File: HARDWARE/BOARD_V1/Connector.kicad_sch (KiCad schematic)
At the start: 40 parts, among them J1 SFW15R-2STE1LF, J2 USB_C_Receptacle_USB2.0_16P, J3 47309-2651, J4 Conn_ARM_SWD_TagConnect_TC203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, J5 687108183722, Q1 BSS84AKQBZ

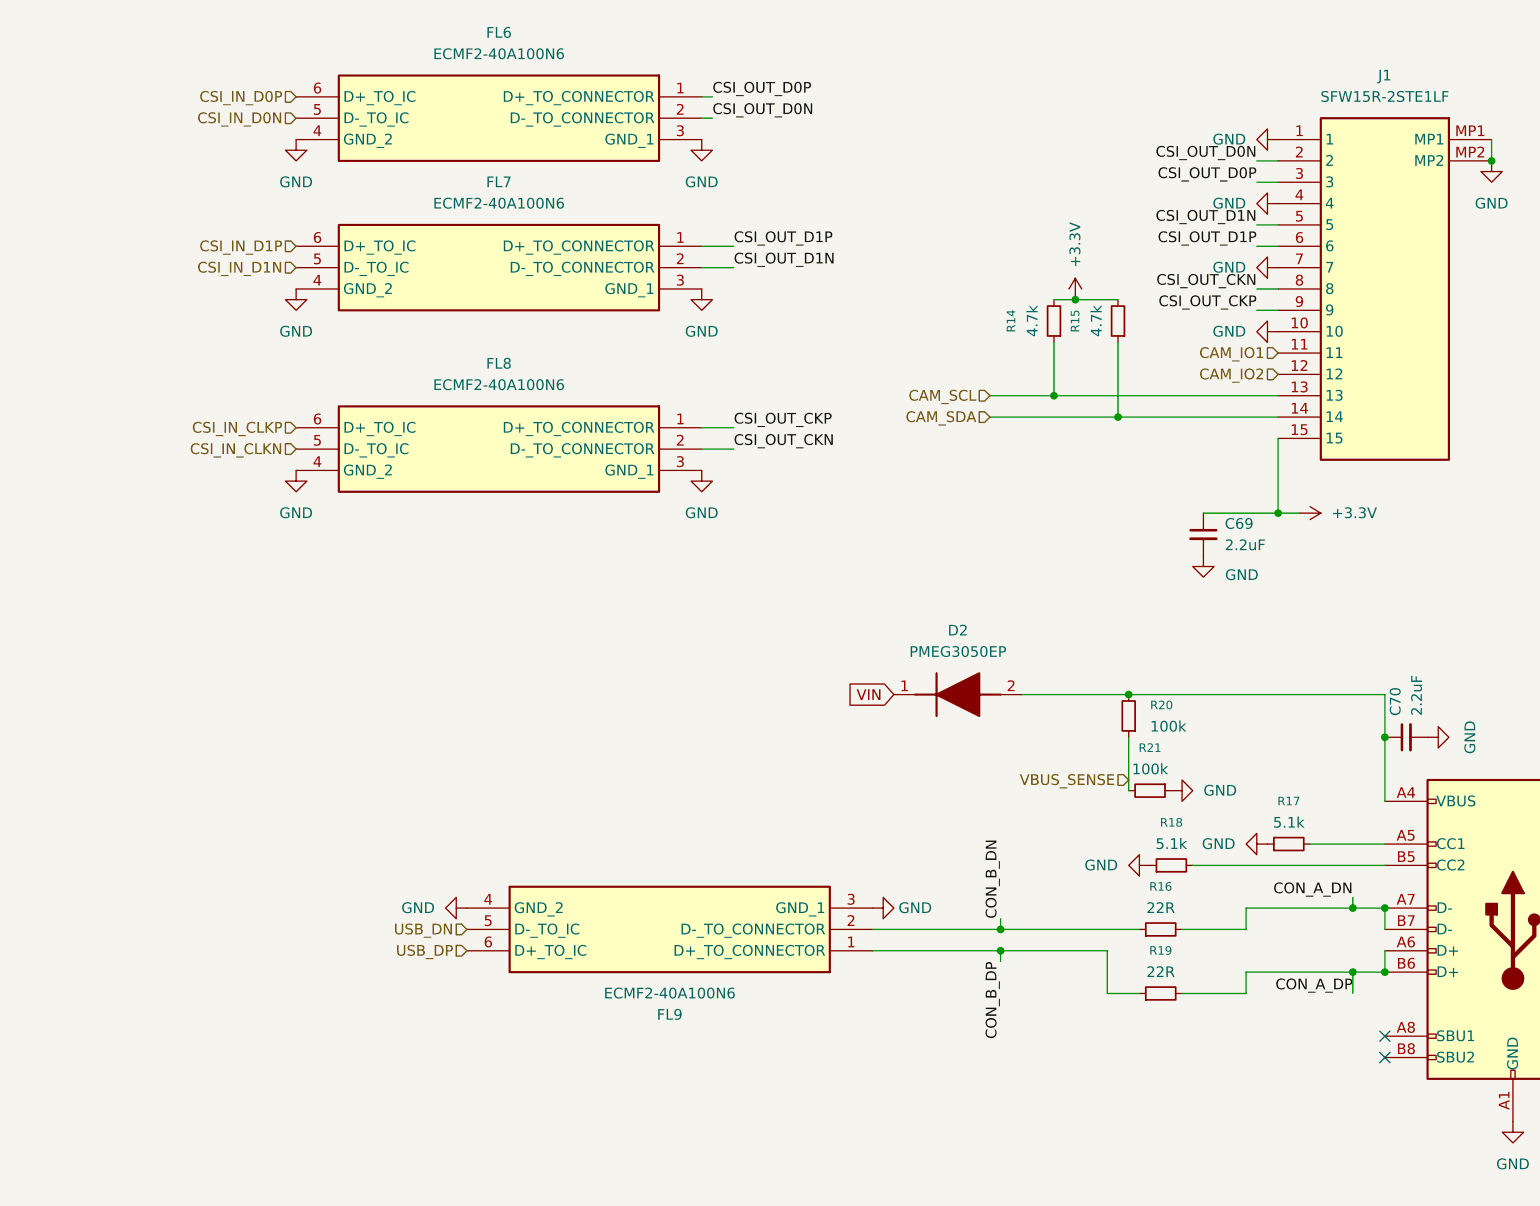
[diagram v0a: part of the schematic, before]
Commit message: up
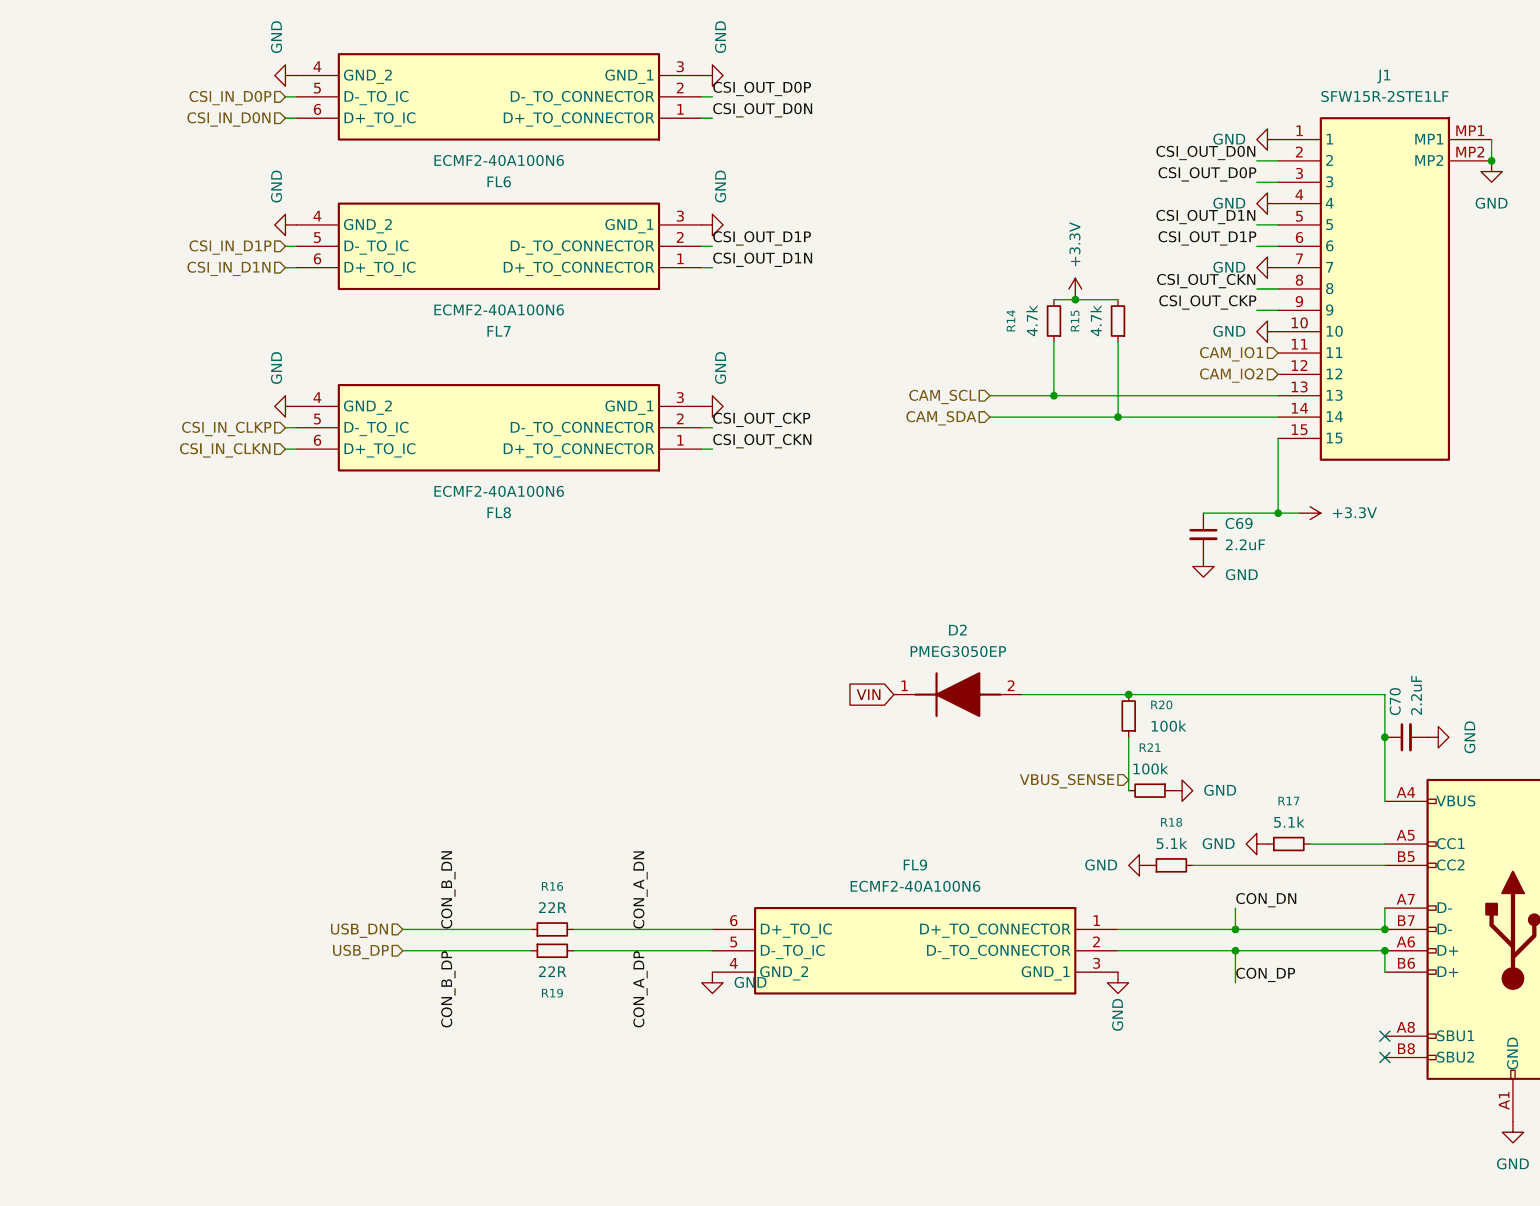
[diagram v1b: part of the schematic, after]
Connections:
- net CON_A_DN: now also FL9.6 (D+_TO_IC); no longer J2.A7 (D-), J2.B7 (D-)
- net CON_A_DP: now also FL9.5 (D-_TO_IC); no longer J2.A6 (D+), J2.B6 (D+)
- net CSI_IN_CLKN: now also FL8.6 (D+_TO_IC); no longer FL8.5 (D-_TO_IC)
- net CSI_IN_CLKP: now also FL8.5 (D-_TO_IC); no longer FL8.6 (D+_TO_IC)
- net CSI_IN_D0N: now also FL6.6 (D+_TO_IC); no longer FL6.5 (D-_TO_IC)
- net CSI_IN_D0P: now also FL6.5 (D-_TO_IC); no longer FL6.6 (D+_TO_IC)
- net CSI_IN_D1N: now also FL7.6 (D+_TO_IC); no longer FL7.5 (D-_TO_IC)
- net CSI_IN_D1P: now also FL7.5 (D-_TO_IC); no longer FL7.6 (D+_TO_IC)
- net CSI_OUT_CKN: now also FL8.1 (D+_TO_CONNECTOR); no longer FL8.2 (D-_TO_CONNECTOR)
- net CSI_OUT_CKP: now also FL8.2 (D-_TO_CONNECTOR); no longer FL8.1 (D+_TO_CONNECTOR)
- net CSI_OUT_D0N: now also FL6.1 (D+_TO_CONNECTOR); no longer FL6.2 (D-_TO_CONNECTOR)
- net CSI_OUT_D0P: now also FL6.2 (D-_TO_CONNECTOR); no longer FL6.1 (D+_TO_CONNECTOR)
- net CSI_OUT_D1N: now also FL7.1 (D+_TO_CONNECTOR); no longer FL7.2 (D-_TO_CONNECTOR)
- net CSI_OUT_D1P: now also FL7.2 (D-_TO_CONNECTOR); no longer FL7.1 (D+_TO_CONNECTOR)
- net USB_DN: now also R16.1; no longer FL9.5 (D-_TO_IC)
- net USB_DP: now also R19.1; no longer FL9.6 (D+_TO_IC)
- net CON_B_DN renamed CON_DP
- net CON_DP: now also J2.A6 (D+), J2.B6 (D+); no longer R16.1
- net CON_B_DP renamed CON_DN
- net CON_DN: now also J2.A7 (D-), J2.B7 (D-); no longer R19.1
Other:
- moved on the sheet: FL6, FL7, FL8, FL9
